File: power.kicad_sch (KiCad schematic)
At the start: 32 parts, among them Q401 AO3400A, U301 TPS563201DDCR, U302 AMS1117-3.3

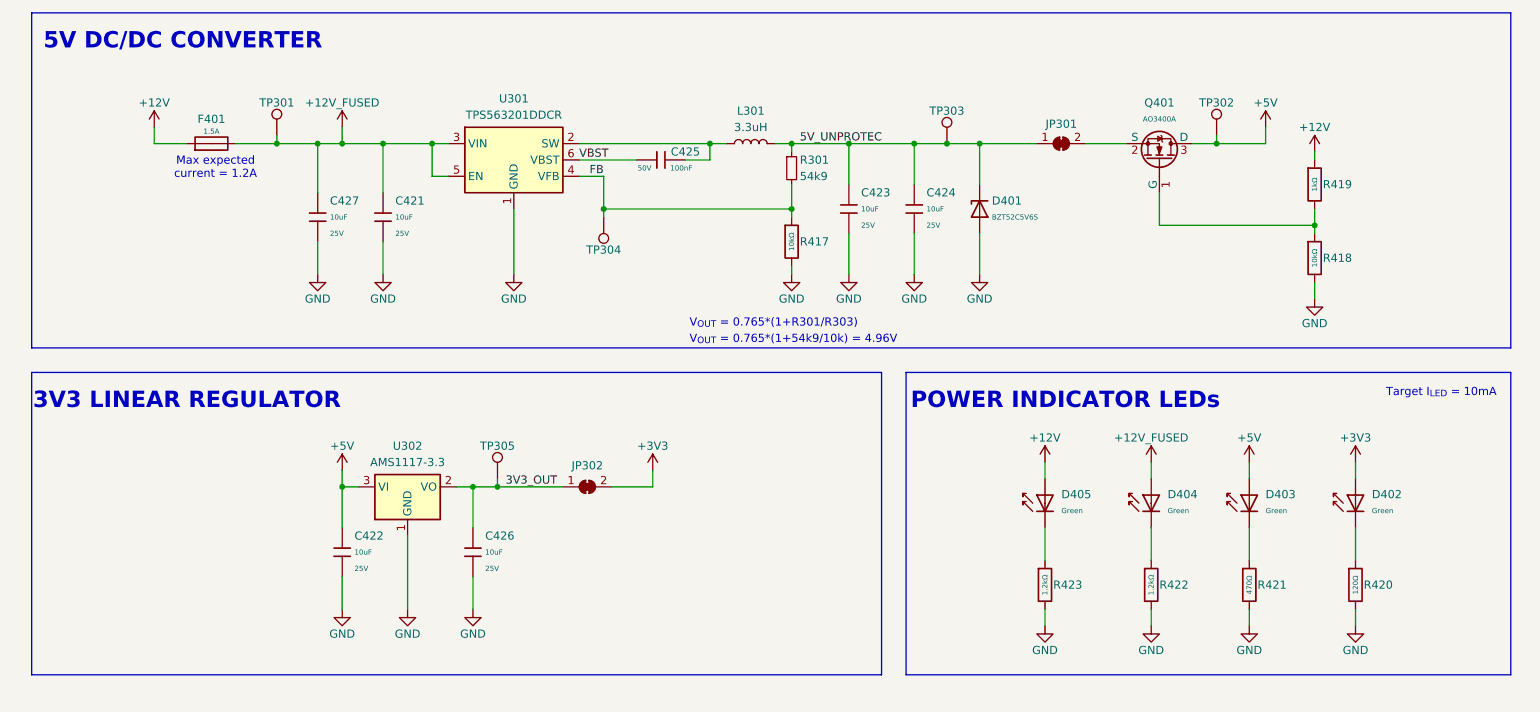
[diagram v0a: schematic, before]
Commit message: [3] Add second converter
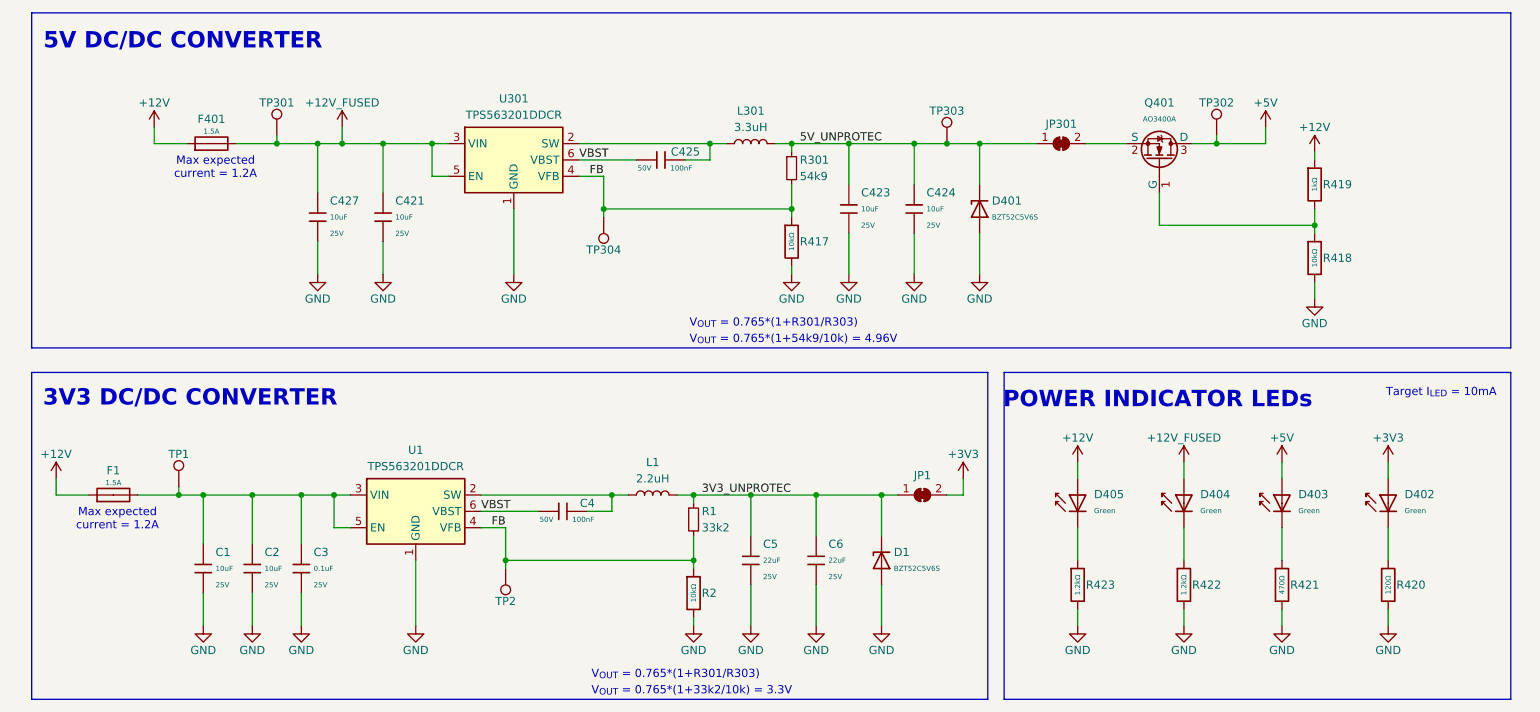
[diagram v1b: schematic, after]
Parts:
- removed C422, C426: 10uF, PCM_JLCPCB:C_0603, symbol PCM_JLCPCB-Capacitors:0603,10uF,(2)
- removed JP302: Test LDO Vout, symbol Jumper:SolderJumper_2_Bridged
- removed TP305: LDO vout, symbol Connector:TestPoint
- removed U302: AMS1117-3.3, Package_TO_SOT_SMD:SOT-223-3_TabPin2, symbol Regulator_Linear:AMS1117-3.3
- added C1, C2: 10uF, PCM_JLCPCB:C_0603, symbol PCM_JLCPCB-Capacitors:0603,10uF,(2)
- added C3: 0.1uF, PCM_JLCPCB:C_0603, symbol PCM_JLCPCB-Capacitors:0603,10uF,(2)
- added C4: 100nF, PCM_JLCPCB:C_0402, symbol PCM_JLCPCB-Capacitors:0402,100nF,(2)
- added C5, C6: 22uF, PCM_JLCPCB:C_0603, symbol PCM_JLCPCB-Capacitors:0603,10uF,(2)
- added D1: BZT52C5V6S, PCM_JLCPCB:D_SOD-323, symbol PCM_JLCPCB-Diodes:Zener,BZT52C5V6S
- added F1: 1.5A, PCM_JLCPCB:F_0603, symbol PCM_JLCPCB-Variable-Resistors:Fuse,1.5A
- added JP1: Test Buck Vout, symbol Jumper:SolderJumper_2_Bridged
- added L1: 2.2uH, symbol Device:L
- added R1: 33k2, symbol Device:R_Small
- added R2: 10kΩ, PCM_JLCPCB:R_0402, symbol PCM_JLCPCB-Resistors:0402,10kΩ
- added TP1: TestPoint, symbol Connector:TestPoint
- added TP2: Buck Feedback, symbol Connector:TestPoint
- added U1: TPS563201DDCR, Package_TO_SOT_SMD:SOT-23-6, symbol Regulator_Switching:TPS563200
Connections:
- net +12V: now also F1.1
- net +3V3: now also JP1.2 (B)
- net FB: now also R1.2, R2.1, TP2.1, U1.4 (VFB)
- net GND: now also C1.2, C2.2, C3.2, C5.2, C6.2, D1.2, R2.2, U1.1 (GND)
- net VBST: now also C4.1, U1.6 (VBST)
- new net: C1.1, C2.1, C3.1, F1.2, TP1.1, U1.3 (VIN), U1.5 (EN)
- new net: C4.2, L1.1, U1.2 (SW)
- new net 3V3_UNPROTEC: C5.1, C6.1, D1.1, JP1.1 (A), L1.2, R1.1
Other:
- note added: "3V3 DC/DC CONVERTER"
- note added: "V_{OUT} = 0.765*(1+33k2/10k) = 3.3V"
- note removed: "3V3 LINEAR REGULATOR"
- moved on the sheet: D402, D403, D404, D405, R420, R421, R422, R423
